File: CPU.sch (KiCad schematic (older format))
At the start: 105 parts, among them J1 Conn_01x30, J2 Conn_01x30, U1 USB_MICRO, U10 GD5F1GQ4UAYIG, U11 EA3036, U12 XC6206, U2 NS2009, U3 FC-40P-LCD, U4 allwinner-V3S-eLQFP128, U5 TF_CARD, U6 MC-146, U7 MX25L12835F, U8 PT4101, U9 XT_3225

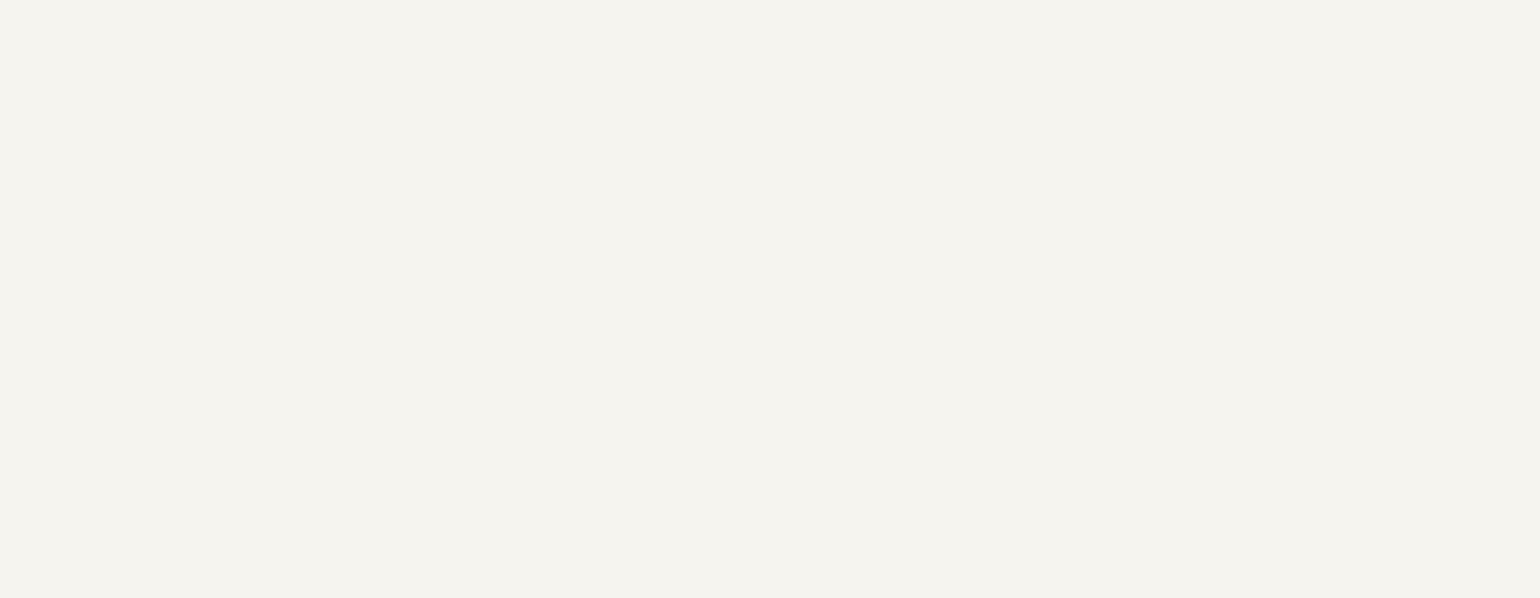
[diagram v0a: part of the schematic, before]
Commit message: update,
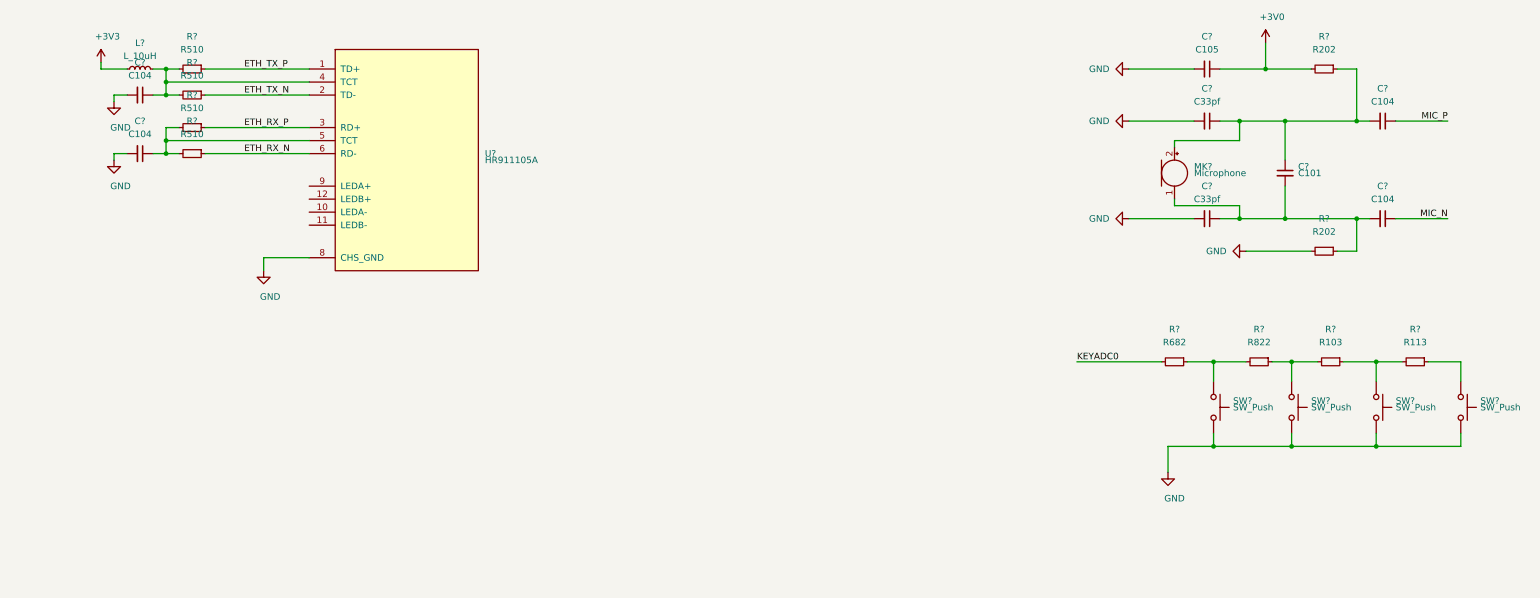
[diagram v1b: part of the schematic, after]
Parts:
- added C? (x4): C104, symbol taobao-c:C104
- added C?: C105, symbol taobao-c:C105
- added C? (x2): C33pf, symbol taobao-c:C33pf
- added C?: C101, symbol taobao-c:C101
- added L?: L_10uH, symbol taobao-l:L_10uH
- added MK?: Microphone, symbol Device:Microphone
- added R? (x4): R510, symbol taobao-r:R510
- added R? (x2): R202, symbol taobao-r:R202
- added R?: R682, symbol taobao-r:R682
- added R?: R822, symbol taobao-r:R822
- added R?: R103, symbol taobao-r:R103
- added R?: R113, symbol taobao-r:R113
- added SW? (x4): SW_Push, symbol Switch:SW_Push
- added U?: HR911105A, footprint-lib.pretty:HANRUN_HR911105A, symbol taobao-components:HR911105A
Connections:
- net +3V0: now also C?.1, R?.2
- net +3V3: now also L?.1
- net ETH_RX_N: now also R?.1, U?.6 (RD-)
- net ETH_RX_P: now also R?.1, U?.3 (RD+)
- net ETH_TX_N: now also R?.1, U?.2 (TD-)
- net ETH_TX_P: now also R?.1, U?.1 (TD+)
- net GND: now also C?.2, C?.2, C?.2, C?.2, C?.2, R?.2, SW?.2, SW?.2, SW?.2, SW?.2, U?.8 (CHS_GND)
- net KEYADC0: now also R?.2
- net MIC_N: now also C?.1
- net MIC_P: now also C?.1
- new net: C?.1, L?.2, R?.2, R?.2, U?.4 (TCT)
- new net: C?.1, R?.2, R?.2, U?.5 (TCT)
- new net: C?.1, C?.2, C?.2, MK?.1 (-), R?.1
- new net: C?.1, C?.1, C?.2, MK?.2 (+), R?.1
- new net: R?.1, R?.2, SW?.1 (x3)
- new net: R?.1, SW?.1
